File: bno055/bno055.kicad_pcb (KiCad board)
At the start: 4 copper layers, 11 parts, among them U1 BNO055, Y1 NX3215SA-32.768K-STD-MUA-14

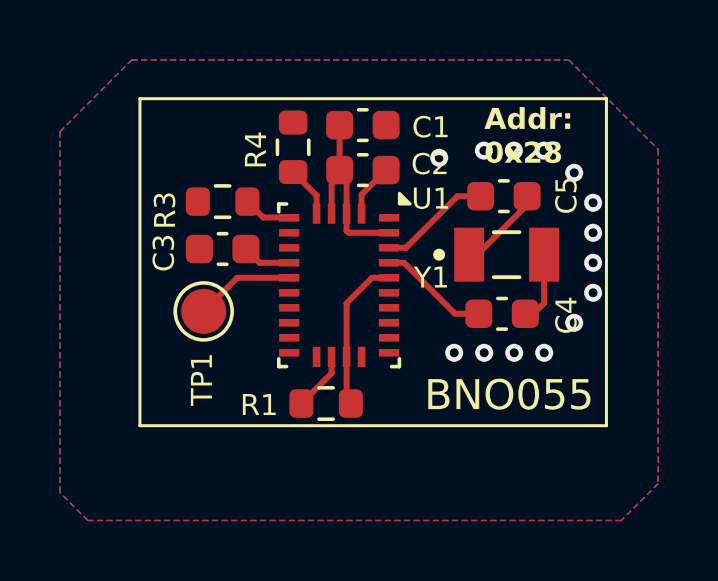
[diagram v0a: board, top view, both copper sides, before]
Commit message: [Rushil] added block of ds3231_rtc
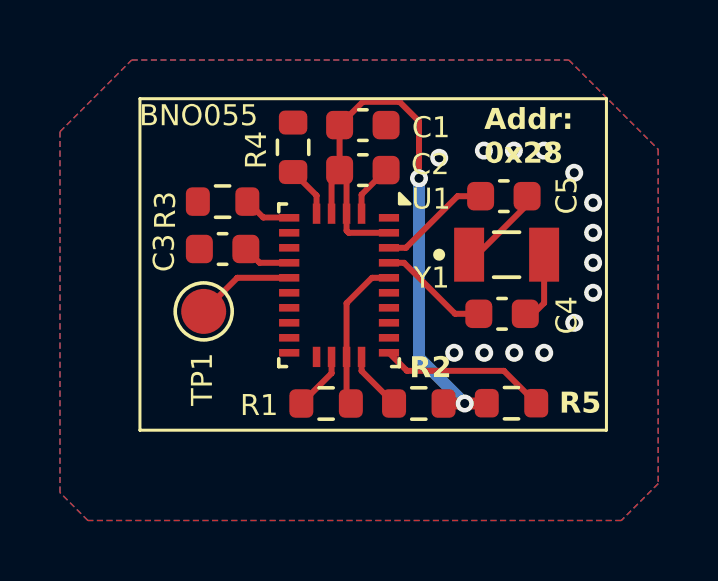
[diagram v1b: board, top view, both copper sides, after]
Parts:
- added R2: 10k, Resistor_SMD:R_0603_1608Metric, F.Cu at (113.8, 78.7)
- added R5: 10k, Resistor_SMD:R_0603_1608Metric, F.Cu at (116.9, 78.7)
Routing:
- net /block_bno055/+3V3: track 6.62 -> 21.3 mm, vias 0 -> 2
- net /block_bno055/SDA: track 0.00 -> 5.61 mm
- net /block_bno055/SCL: track 0.00 -> 2.00 mm
